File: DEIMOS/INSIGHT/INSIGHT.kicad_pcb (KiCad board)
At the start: 4 copper layers, 76.8 x 38.1 mm, 76 parts, among them J1 Batt, J2 SMA-J-P-GF-RA-SM1, J3 USB_C_Receptacle_USB2.0_16P, J4 Boot, J5 GND, SW3 SW_SPDT, U1 LSM6DS3, U2 MPL3115A2, U3 W25Q128JVSIQ, U4 BNO085, U5 RP2040, U6 Adafruit GPS, U7 MPM3610GQV-Z, U8 RFM95W-915S2, Y1 ABM8-272-T3, Y2 ABS07-32.768KHZ-1-T

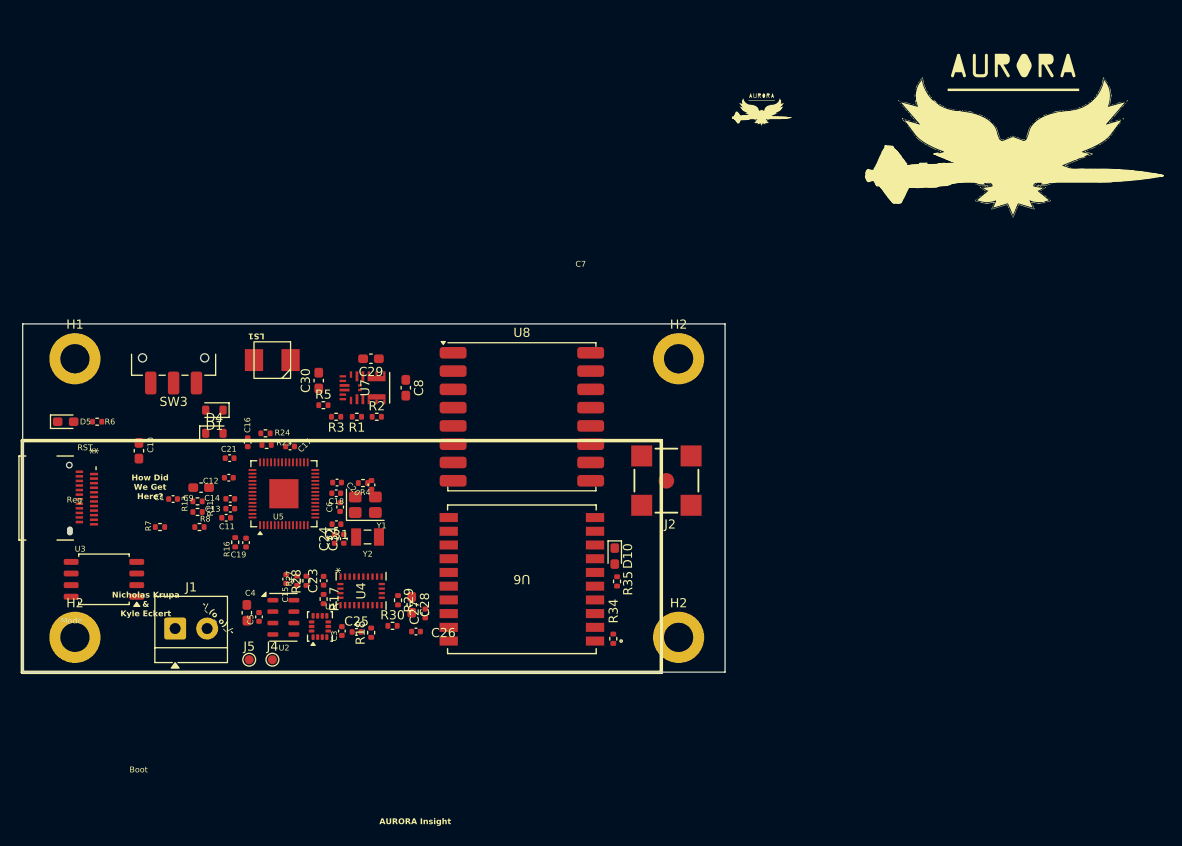
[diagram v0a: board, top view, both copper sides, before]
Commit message: Centered eveyrhting
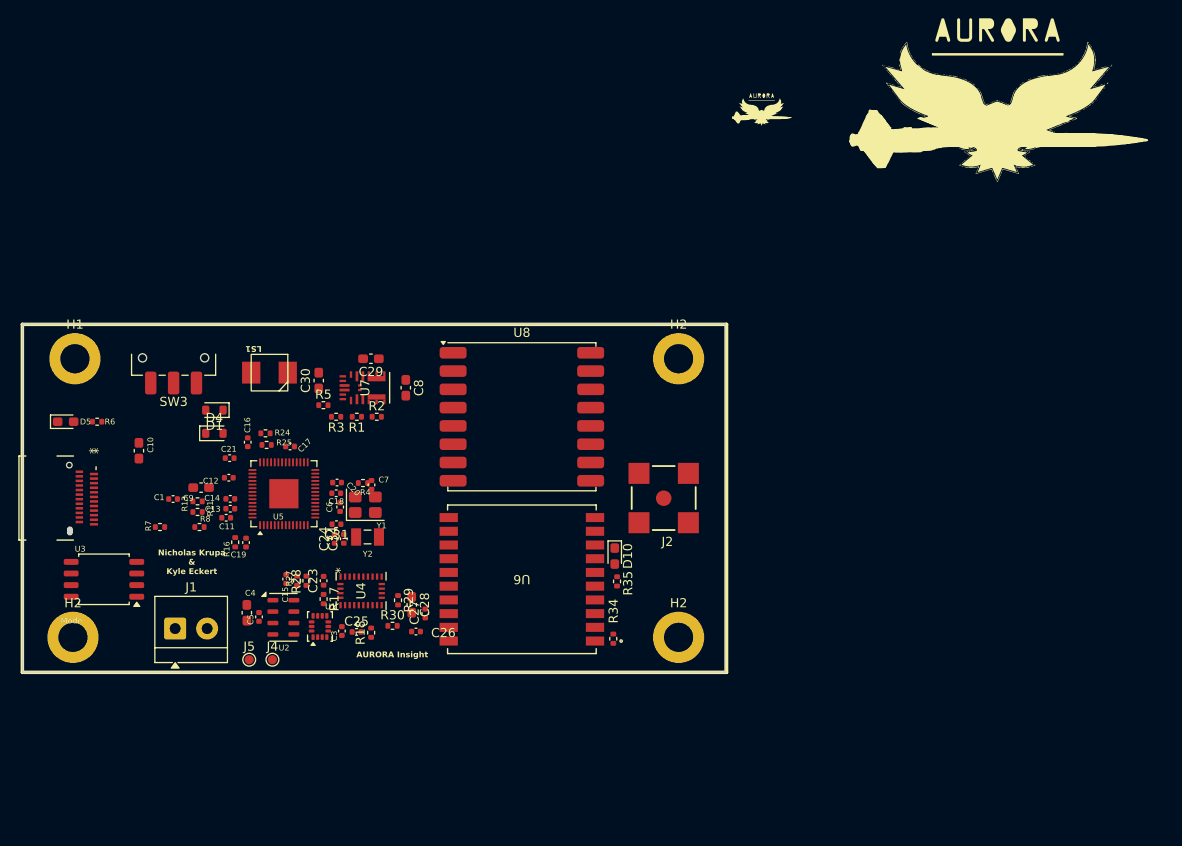
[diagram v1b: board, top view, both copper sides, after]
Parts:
- moved J2 1.93 mm to (137.4, 67.1)
- moved LS1 1.41 mm to (94.3, 50.1)
- moved H2 0.22 mm to (72.8, 82.4)
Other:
- board text removed: "-\_(o_o)_/-"
- board text removed: "Boot"
- board text removed: "How Did We Get Here?"
- board text removed: "RST"
- board text removed: "Reg"
